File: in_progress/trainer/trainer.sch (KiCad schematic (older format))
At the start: 23 parts

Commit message: .
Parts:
- C? (x2): symbol C -> C-RESCUE-trainer
- Q?: symbol PN2222A -> PN2222A-RESCUE-trainer
- R? (x5): symbol R -> R-RESCUE-trainer
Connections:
- wire segments 61 -> 52
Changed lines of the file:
@@
 LIBS:memory
 LIBS:xilinx
-LIBS:special
 LIBS:microcontrollers
 LIBS:dsp
@@
 LIBS:valves
 LIBS:MiscellaneousDevices
+LIBS:ULN280xA
 LIBS:Gajda_cmosieee
 LIBS:jhd-162a
 LIBS:capteurs
 LIBS:trainer-cache
-EELAYER 27 0
+EELAYER 25 0
 EELAYER END
 $Descr A4 11693 8268
@@
 $EndComp
 $Comp
-L C C?
+L C-RESCUE-trainer C?
 U 1 1 5657DDA5
 P 2100 2900
@@
 $EndComp
 $Comp
-L C C?
+L C-RESCUE-trainer C?
 U 1 1 5657DE9C
 P 2900 2900
@@
 $EndComp
 $Comp
-L R R?
+L R-RESCUE-trainer R?
 U 1 1 5659DCCE
 P 3250 4800
@@
 $EndComp
 $Comp
-L R R?
+L R-RESCUE-trainer R?
 U 1 1 5659E1A6
 P 3250 4900
@@
 $EndComp
 $Comp
-L R R?
+L R-RESCUE-trainer R?
 U 1 1 5659E1E3
 P 3250 5000
@@
 $EndComp
 $Comp
-L R R?
+L R-RESCUE-trainer R?
 U 1 1 5659E227
 P 3250 5100
@@
 	2900 2750 2900 2650
 Wire Wire Line
-	2900 2650 3250 2650
-Wire Wire Line
-	3250 2650 3500 2650
+	2900 2650 3500 2650
 Wire Wire Line
 	2100 2650 2100 2750
@@
 	3250 2650 3250 2500
 Wire Wire Line
-	1650 2750 1650 2850
-Wire Wire Line
-	1650 2850 1650 3100
+	1650 2750 1650 3100
 Connection ~ 1650 2850
 Wire Wire Line
-	1650 3100 2100 3100
-Wire Wire Line
-	2100 3100 2500 3100
-Wire Wire Line
-	2500 3100 2900 3100
-Wire Wire Line
-	2900 3100 3500 3100
+	1650 3100 3500 3100
 Wire Wire Line
 	2900 3100 2900 3050
 Wire Wire Line
-	2500 2950 2500 3100
-Wire Wire Line
-	2500 3100 2500 3200
+	2500 2950 2500 3200
 Connection ~ 2900 3100
 Connection ~ 2500 3100
@@
 	3000 5100 3100 5100
 Wire Wire Line
-	4000 3950 4000 4200
-Wire Wire Line
-	4000 4200 4000 5000
-Wire Wire Line
-	4000 5000 4000 5800
-Wire Wire Line
-	4000 5800 4000 6600
+	4000 3950 4000 6600
 Wire Wire Line
 	4000 4200 4200 4200
@@
 	8650 3450 8650 3850
 $Comp
-L PN2222A Q?
+L PN2222A-RESCUE-trainer Q?
 U 1 1 565B1B0C
 P 8750 4250
@@
 	8650 4450 8650 4550
 $Comp
-L R R?
+L R-RESCUE-trainer R?
 U 1 1 565B1BAF
 P 9400 4250

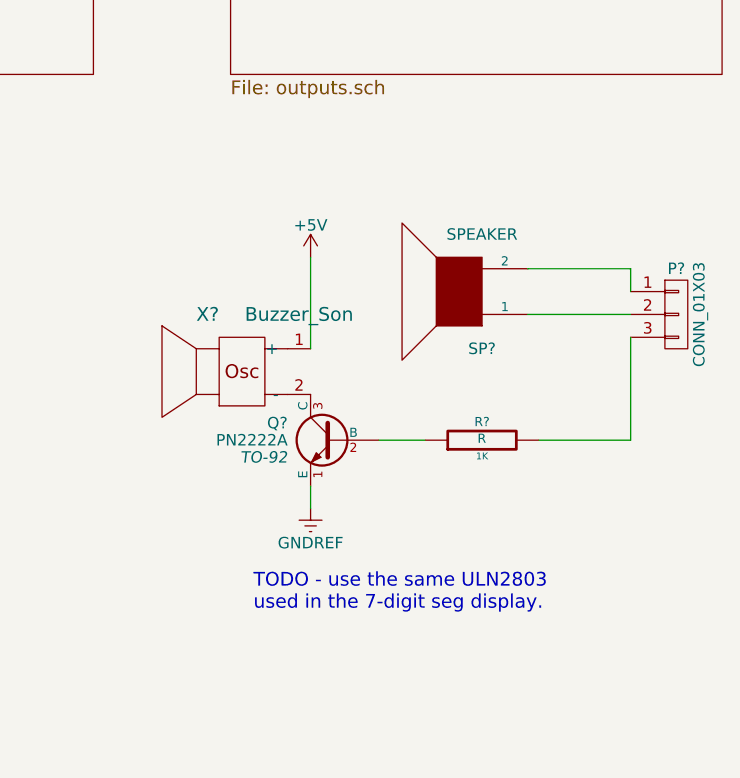
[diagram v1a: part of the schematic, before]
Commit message: .
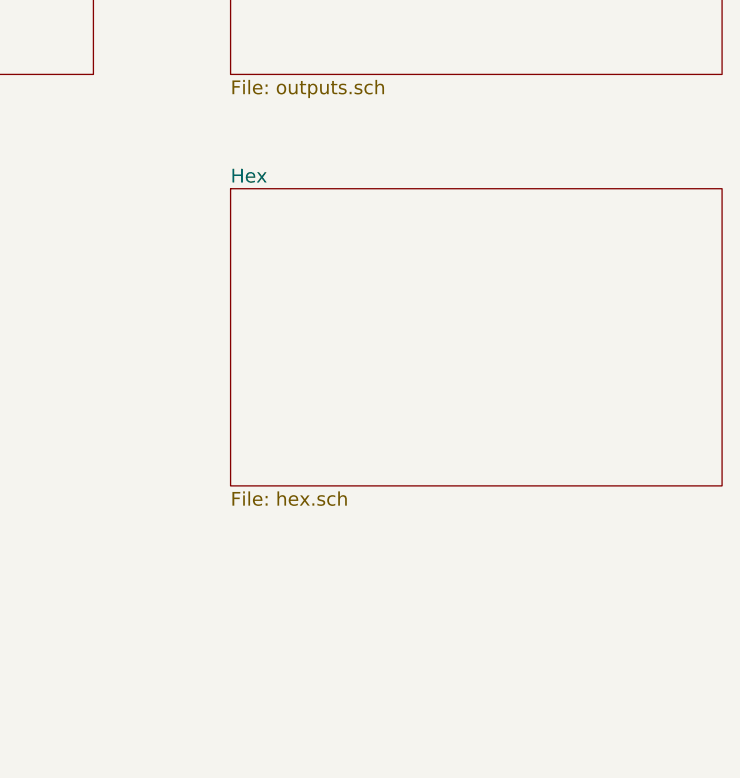
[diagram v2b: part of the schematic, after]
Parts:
- removed P?: CONN_01X03, symbol CONN_01X03
- removed Q?: PN2222A, TO-92, symbol PN2222A-RESCUE-trainer
- removed R?: R, 1K, symbol R-RESCUE-trainer
- removed SP?: SPEAKER, symbol SPEAKER
- removed X?: Buzzer_Son, symbol Buzzer_Son
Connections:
- wire segments 52 -> 44
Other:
- note removed: "TODO - use the same ULN2803 \nused in the 7-digit seg display."
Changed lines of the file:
@@
 $Descr A4 11693 8268
 encoding utf-8
-Sheet 1 3
+Sheet 1 4
 Title ""
 Date "29 nov 2015"
@@
 Text Notes 1800 3650 0    60   ~ 0
 Isolated power supply\n(powers internal LEDs, ICs)
-$Comp
-L CONN_01X03 P?
-U 1 1 565A63D3
-P 10250 3700
-F 0 "P?" H 10250 3900 50  0000 C CNN
-F 1 "CONN_01X03" V 10350 3700 50  0000 C CNN
-F 2 "" H 10250 3700 60  0000 C CNN
-F 3 "" H 10250 3700 60  0000 C CNN
-	1    10250 3700
-	1    0    0    -1
-$EndComp
-$Comp
-L SPEAKER SP?
-U 1 1 565A67F9
-P 9300 3600
-F 0 "SP?" H 9200 3850 50  0000 C CNN
-F 1 "SPEAKER" H 9200 3350 50  0000 C CNN
-F 2 "" H 9300 3600 60  0000 C CNN
-F 3 "" H 9300 3600 60  0000 C CNN
-	1    9300 3600
-	-1   0    0    1
-$EndComp
-$Comp
-L Buzzer_Son X?
-U 1 1 565A69C0
-P 8350 3950
-F 0 "X?" H 8200 4200 60  0000 C CNN
-F 1 "Buzzer_Son" H 8600 4200 60  0000 C CNN
-F 2 "" H 8350 3950 60  0000 C CNN
-F 3 "" H 8350 3950 60  0000 C CNN
-	1    8350 3950
-	1    0    0    -1
-$EndComp
-Wire Wire Line
-	10050 3700 9600 3700
-Wire Wire Line
-	9600 3500 10050 3500
-Wire Wire Line
-	10050 3500 10050 3600
-$Comp
-L +5V #PWR?
-U 1 1 565B1AC3
-P 8650 3450
-F 0 "#PWR?" H 8650 3300 50  0001 C CNN
-F 1 "+5V" H 8650 3590 50  0000 C CNN
-F 2 "" H 8650 3450 60  0000 C CNN
-F 3 "" H 8650 3450 60  0000 C CNN
-	1    8650 3450
-	1    0    0    -1
-$EndComp
-Wire Wire Line
-	8650 3450 8650 3850
-$Comp
-L PN2222A-RESCUE-trainer Q?
-U 1 1 565B1B0C
-P 8750 4250
-F 0 "Q?" H 8950 4325 50  0000 L CNN
-F 1 "PN2222A" H 8950 4250 50  0000 L CNN
-F 2 "TO-92" H 8950 4175 50  0000 L CIN
-F 3 "" H 8750 4250 50  0000 L CNN
-	1    8750 4250
-	-1   0    0    -1
-$EndComp
-$Comp
-L GNDREF #PWR?
-U 1 1 565B1B2B
-P 8650 4550
-F 0 "#PWR?" H 8650 4300 50  0001 C CNN
-F 1 "GNDREF" H 8650 4400 50  0000 C CNN
-F 2 "" H 8650 4550 60  0000 C CNN
-F 3 "" H 8650 4550 60  0000 C CNN
-	1    8650 4550
-	1    0    0    -1
-$EndComp
-Wire Wire Line
-	8650 4450 8650 4550
-$Comp
-L R-RESCUE-trainer R?
-U 1 1 565B1BAF
-P 9400 4250
-F 0 "R?" V 9480 4250 40  0000 C CNN
-F 1 "R" V 9407 4251 40  0000 C CNN
-F 2 "1K" V 9330 4250 30  0000 C CNN
-F 3 "~" H 9400 4250 30  0000 C CNN
-	1    9400 4250
-	0    -1   -1   0
-$EndComp
-Wire Wire Line
-	8950 4250 9150 4250
-Wire Wire Line
-	9650 4250 10050 4250
-Wire Wire Line
-	10050 4250 10050 3800
-Text Notes 8400 5000 0    60   ~ 0
-TODO - use the same ULN2803 \nused in the 7-digit seg display.
+$Sheet
+S 8300 3150 2150 1300
+U 565EDE3C
+F0 "Hex" 60
+F1 "hex.sch" 60
+$EndSheet
 $EndSCHEMATC
